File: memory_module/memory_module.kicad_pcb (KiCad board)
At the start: 2 copper layers, 100 x 100 mm, 93 parts, among them J1 Conn_01x06_Pin, J2 Conn_01x08_Pin, SW1 SW_DIP_x08, SW2 SW_DIP_x08, SW3 SW_DIP_x08, SW4 SW_DIP_x08, SW5 SW_DIP_x08, SW6 SW_DIP_x08, SW7 SW_DIP_x08, SW8 SW_DIP_x08, U1 74HC138, U2 74HC540

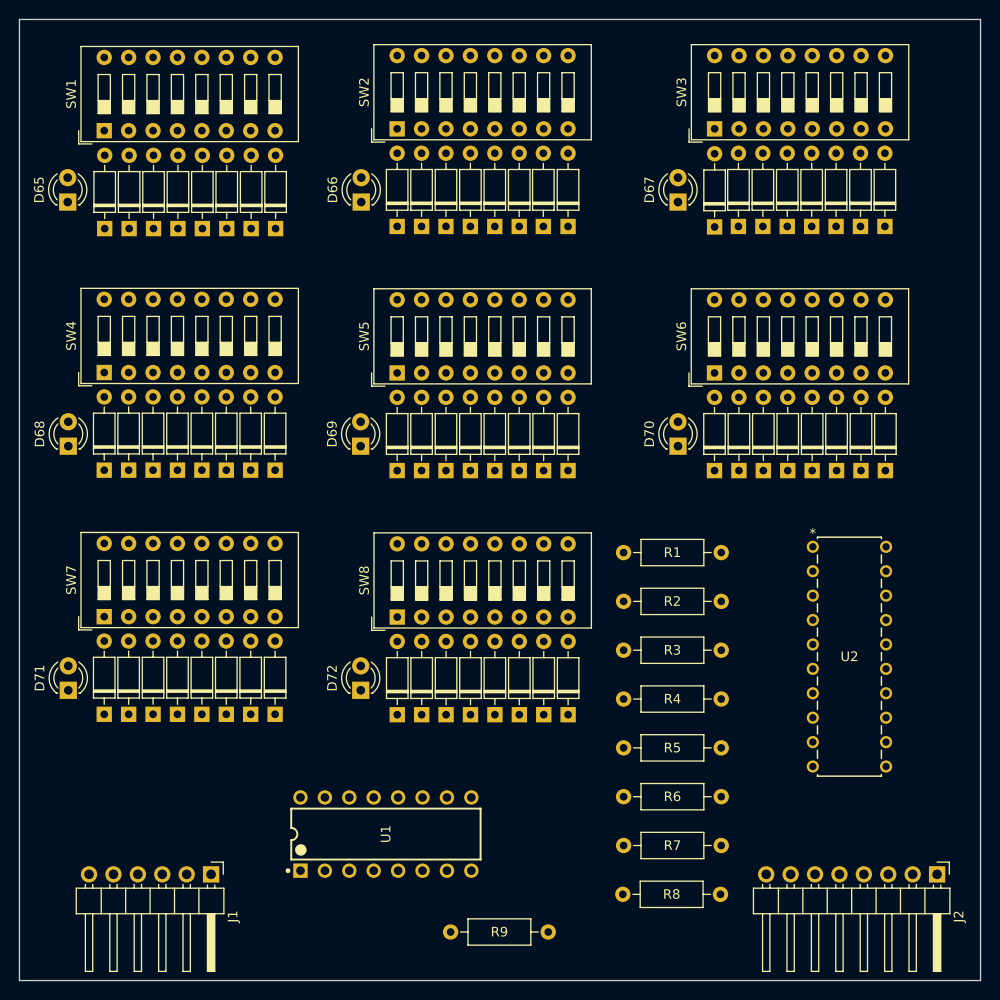
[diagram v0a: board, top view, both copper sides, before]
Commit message: フットプリント位置調整
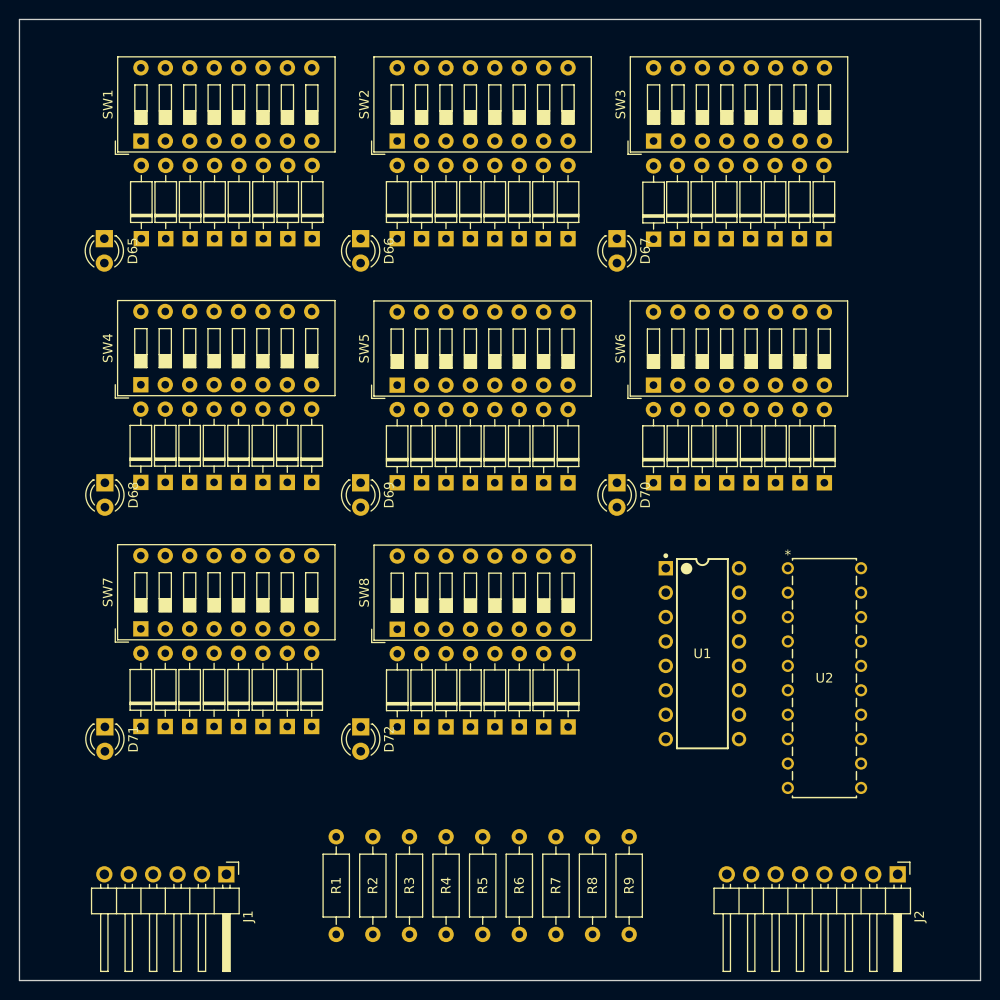
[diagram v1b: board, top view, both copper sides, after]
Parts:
- moved R1 49.8 mm to (73.0, 125.1), turned to -90 degrees
- moved R2 43.7 mm to (76.8, 125.1), turned to -90 degrees
- moved U1 37.9 mm to (111.1, 106.0), turned to 0 degrees
- moved R3 37.8 mm to (80.6, 125.1), turned to -90 degrees
- moved R4 32.0 mm to (84.5, 125.1), turned to -90 degrees
- moved R5 26.5 mm to (88.3, 125.1), turned to -90 degrees
- moved R6 21.4 mm to (92.1, 125.1), turned to -90 degrees
- moved R7 17.2 mm to (95.9, 125.1), turned to -90 degrees
- moved R8 14.6 mm to (99.7, 125.1), turned to -90 degrees
- moved R9 13.0 mm to (103.5, 125.1), turned to -90 degrees
- moved D67 7.41 mm to (102.2, 62.9), turned to -90 degrees
- moved D70 7.41 mm to (102.2, 88.3), turned to -90 degrees
- moved D42 6.48 mm to (108.6, 88.3)
- moved D45 6.48 mm to (116.2, 88.3)
- moved D47 6.48 mm to (121.3, 88.3)
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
